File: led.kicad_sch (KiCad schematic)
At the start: 16 parts

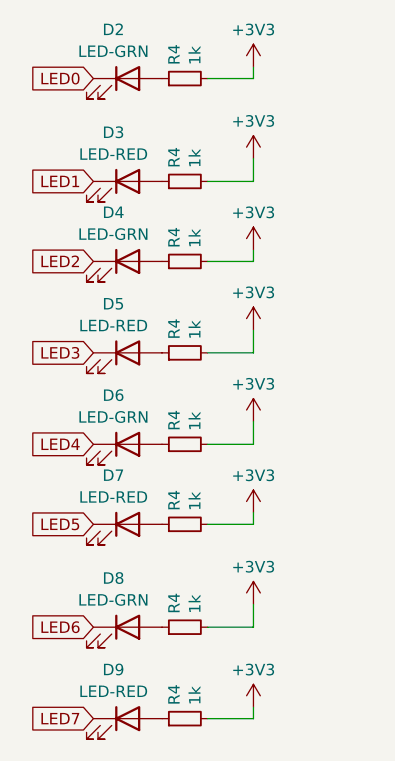
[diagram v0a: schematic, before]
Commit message: Added GPS receiver; increased board size
including battery supply; made board bigger
and added edge connectors for ETH GPIO, PPS
and antenna.
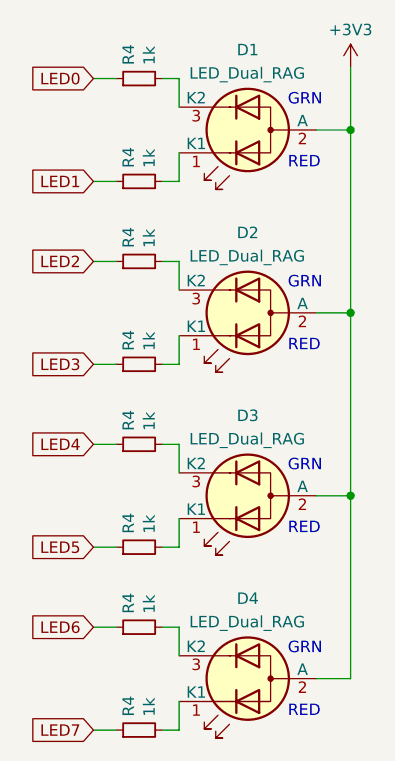
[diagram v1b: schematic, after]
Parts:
- removed D2, D4, D6, D8: LED-GRN, LED_SMD:LED_0603_1608Metric, symbol Device:LED
- removed D3, D5, D7, D9: LED-RED, LED_SMD:LED_0603_1608Metric, symbol Device:LED
- added D1, D2, D3, D4: LED_Dual_RAG, proj_footprints:LED_Wuerth_Sideview, symbol Device:LED_Dual_KAK
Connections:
- net +3V3: now also D1.2 (A), D2.2 (A), D3.2 (A), D4.2 (A); no longer R4.2, R4.2, R4.2, R4.2, R4.2, R4.2, R4.2, R4.2
- net LED0: now also R4.1
- net LED1: now also R4.1
- net LED2: now also R4.1
- net LED3: now also R4.1
- net LED4: now also R4.1
- net LED5: now also R4.1
- net LED6: now also R4.1
- net LED7: now also R4.1
- new net: D1.1 (K1), R4.2
- new net: D1.3 (K2), R4.2
- new net: D3.3 (K2), R4.2
- new net: D4.1 (K1), R4.2
- new net: D4.3 (K2), R4.2
- new net: D2.3 (K2), R4.2
- new net: D2.1 (K1), R4.2
- new net: D3.1 (K1), R4.2
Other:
- note added: "GRN"
- note added: "RED"
- moved on the sheet: R4
